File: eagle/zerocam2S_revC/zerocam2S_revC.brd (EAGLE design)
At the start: 30 x 65 mm, 60 parts, among them IC1 MCP170312MB, J5 CORTEX_DEBUG_PTH, SW1 KSS221GLFS, U1 ATSAMD21G-A, U3 MP2307, X2 ZX62D-B-5PA8, Y2 32.768kHz

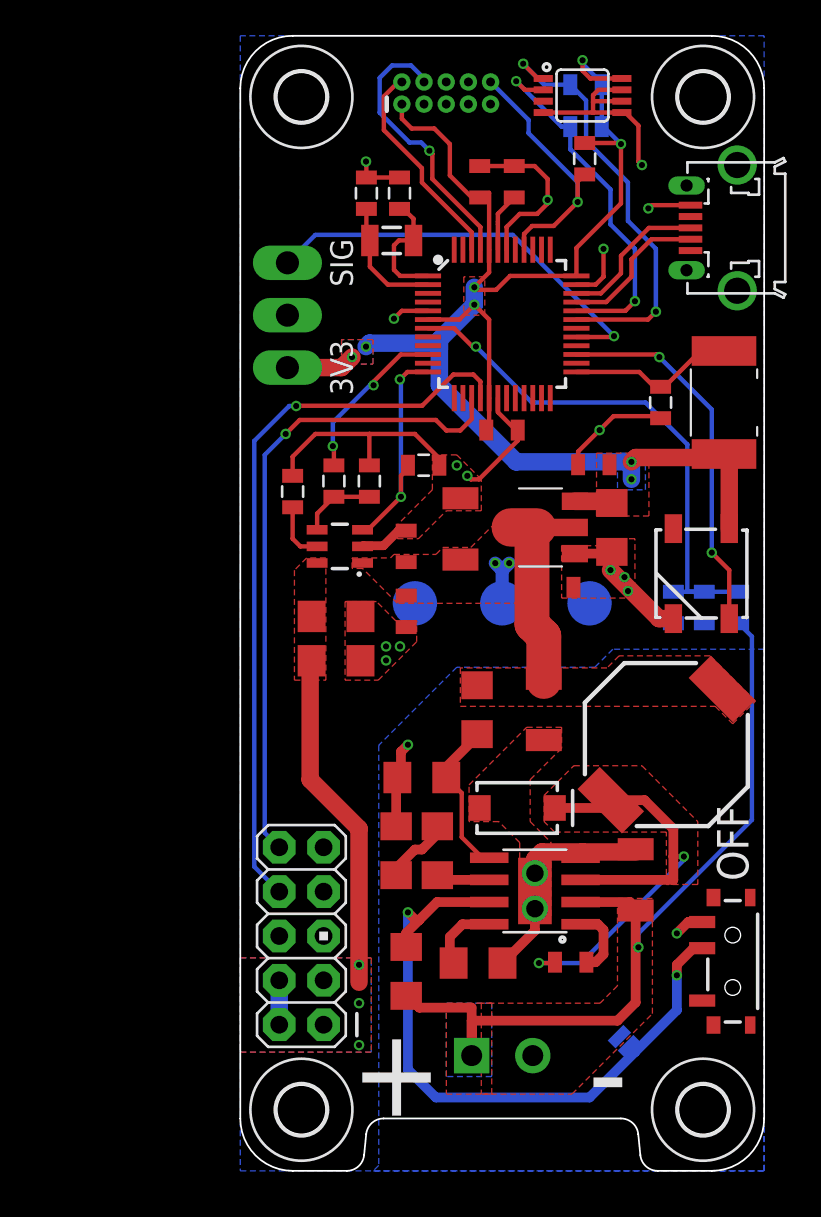
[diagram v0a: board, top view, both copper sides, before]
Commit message: various uncommitted files
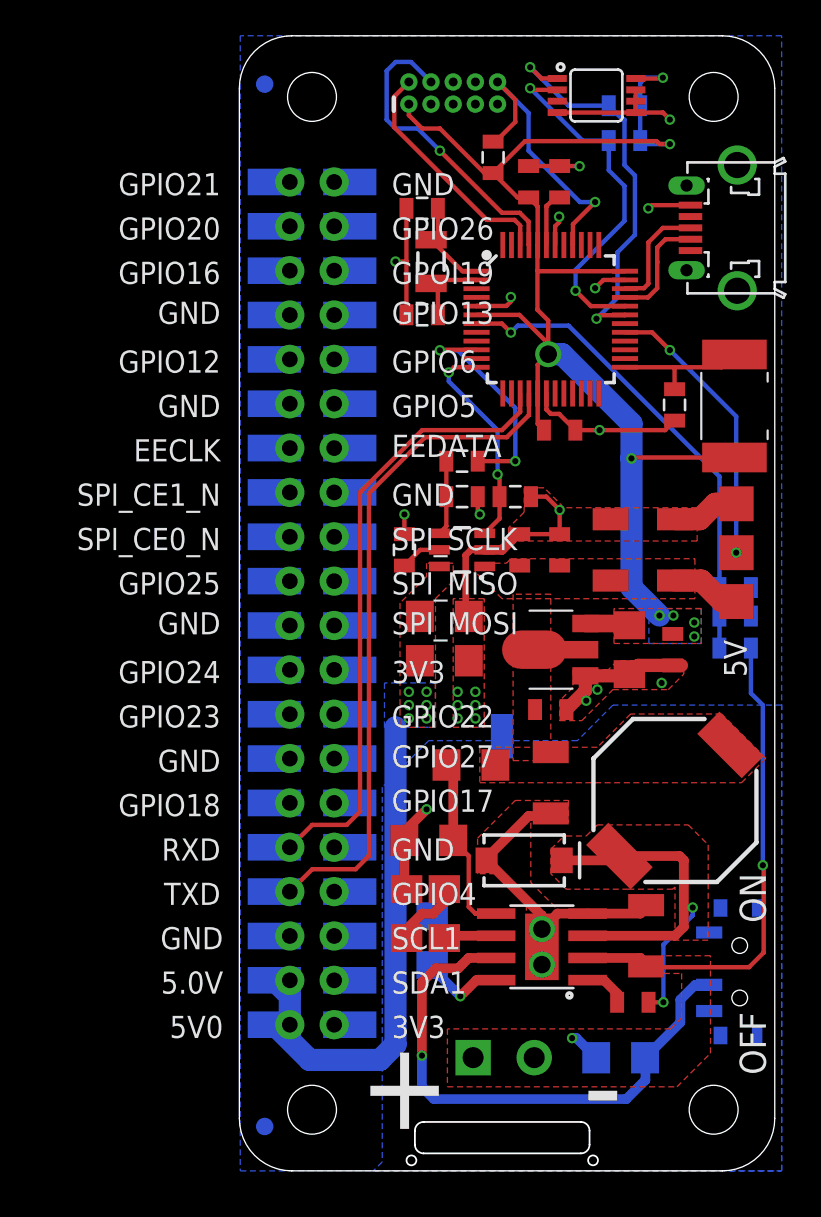
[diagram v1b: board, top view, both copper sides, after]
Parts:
- removed D2: (no value), SparkFun-LED:WS2812B
- removed H1, H2, H3, H4: MOUNT-HOLE2.8, holes:2,8
- removed J2: (no value), SparkFun-Connectors:AVR_ICSP
- removed JP1: JUMPER-SMT_2_NO_NO-SILK, SparkFun-Jumpers:SMT-JUMPER_2_NO_NO-SILK
- removed TP4, TP5, TP6: TPB2,54, testpad:B2,54
- added C22: 100uF, SparkFun-Capacitors:1210
- added RPI1: RASPBERRYPI_BPLUS_BONNET_THMSMT, microbuilder:PI_BONNET_THMSMT
- TP1, TP2, TP3: value TPPAD1-13Y -> TPTP20SQ; device testpad:P1-13Y -> testpad:TP20SQ
- moved TP3 30.6 mm to (28.4, 35.4), turned to 0 degrees
- moved TP1 29.0 mm to (28.4, 32.6), turned to 0 degrees
- moved TP2 27.9 mm to (28.4, 38.2), turned to 0 degrees
- moved R24 13.2 mm to (21.8, 6.47), flipped to the bottom, turned to 180 degrees
- moved C18 11.5 mm to (24.8, 29.8), turned to 270 degrees
- moved C10 9.47 mm to (18.3, 35.6), turned to 90 degrees
- moved C21 8.68 mm to (21.2, 35.6)
- moved C5 7.66 mm to (10.4, 49.0), turned to 0 degrees
- moved R_MOSFET_USB4 7.43 mm to (12.7, 40.6), turned to 0 degrees
- moved R_MOSFET_USB1 7.22 mm to (9.40, 35.6)
- moved C17 7.07 mm to (22.3, 29.8)
- moved IC1 7.03 mm to (17.8, 29.8)
- moved C16 7.01 mm to (17.8, 26.4)
- moved AP2553 7.00 mm to (12.7, 35.6)
- moved C11 6.51 mm to (16.0, 35.6)
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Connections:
- removed net LED: D2.4, U1.27
- net CONV_5V: now also C22.1, TP1.TP; no longer TP4.TP
- net GND: now also C22.2, RPI1.14, RPI1.20, RPI1.25, RPI1.30, RPI1.34, RPI1.39, RPI1.6, RPI1.9, RPI1.S14, RPI1.S20, RPI1.S25, RPI1.S30, RPI1.S34, RPI1.S39, RPI1.S6, RPI1.S9; no longer D2.3, J2.6, J2.9, TP5.TP, TP6.TP
- net GNDA: no longer JP1.2
- net PB_BUCK_EN: no longer JP1.1
- net PI_RX: now also RPI1.10, RPI1.S10; no longer J2.10
- net PI_TX: now also RPI1.8, RPI1.S8; no longer J2.8
- net USB1_OUT: now also RPI1.2, RPI1.4, RPI1.S2, RPI1.S4; no longer J2.2, J2.4
- net VCC: no longer D2.1, TP1.TP
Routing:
- net LED: track 21.4 -> 0.00 mm, vias 2 -> 0
- net BATT_VCC: track 49.2 -> 30.7 mm, vias 1 -> 2
- net CONV_5V: track 16.5 -> 4.01 mm, vias 2 -> 0
- net VCC: track 92.7 -> 80.8 mm
- net USB1_OUT: track 22.1 -> 31.0 mm, vias 3 -> 6
- net SERVO_SIG: track 23.9 -> 16.2 mm, vias 1 -> 2
- net PB_BUCK_EN: track 39.1 -> 31.8 mm, vias 2 -> 1
- net GND: track 69.2 -> 62.5 mm, vias 15 -> 20
- net N$26: track 28.4 -> 23.7 mm
- net GNDA: track 19.0 -> 22.8 mm, vias 2 -> 1
- net VD_DIRECT: track 31.0 -> 27.7 mm
- net USB_FAULT: track 9.70 -> 13.0 mm
- net PI_TX: track 42.0 -> 39.3 mm, vias 1 -> 0
- net N$32: track 7.14 -> 4.82 mm
- net N$27: track 4.78 -> 2.51 mm
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- removed copper zone on layer 16, net BATT_VCC
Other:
- board size 30 x 65 mm -> 30.7 x 65 mm
- board text added: "ON"
- board text added: "rev. C"
- board text added: "zerocam2S1P"
- board text removed: "3V3"
- board text removed: "SIG"
- board text removed: "rev. E"
- board text removed: "zerocam2S"
